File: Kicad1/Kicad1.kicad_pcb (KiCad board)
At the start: 2 copper layers, 12 parts, among them J5 ESP_CONN, J6 ENCODER_CONN, J7 Conn_01x04, U1 STM32F401RBTx, U2 LD1117S50TR_SOT223, U3 LD1117S33TR_SOT223, U4 TB6612FNG, Y1 Crystal_GND24

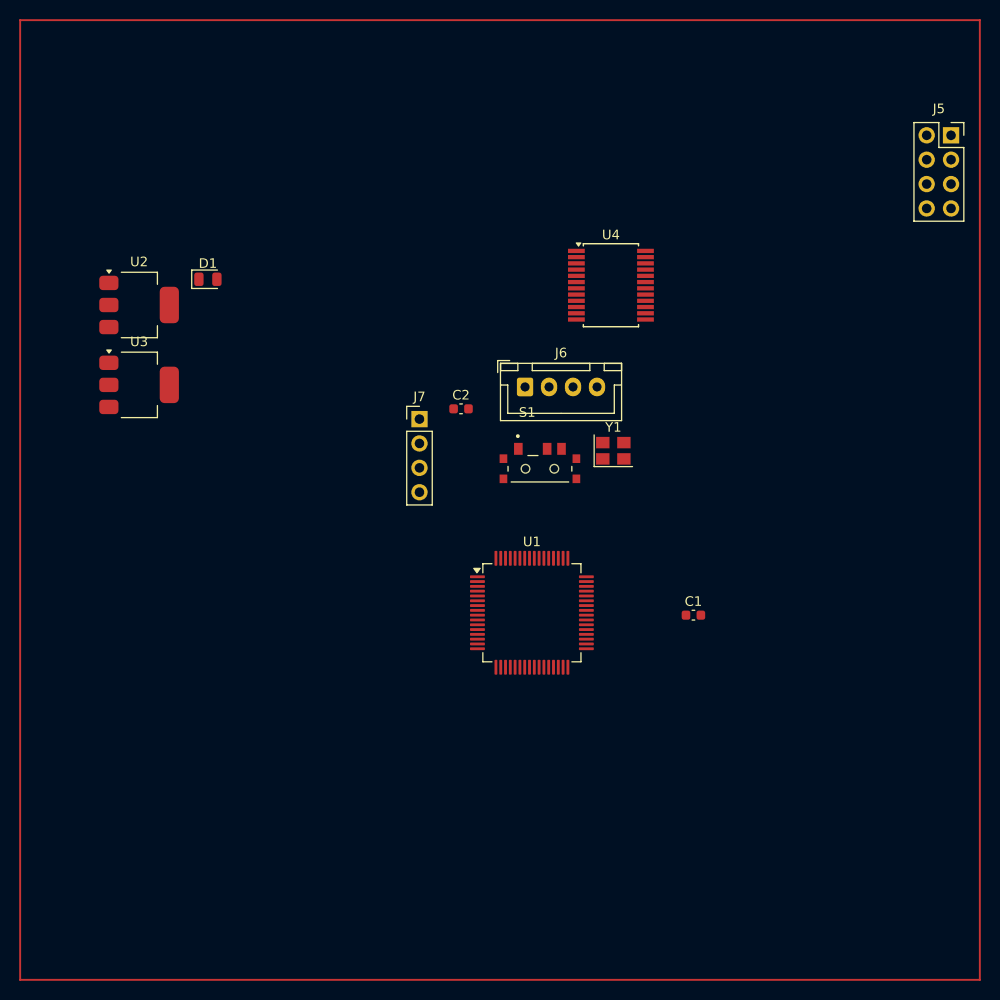
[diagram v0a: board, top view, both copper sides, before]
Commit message: Add files via upload
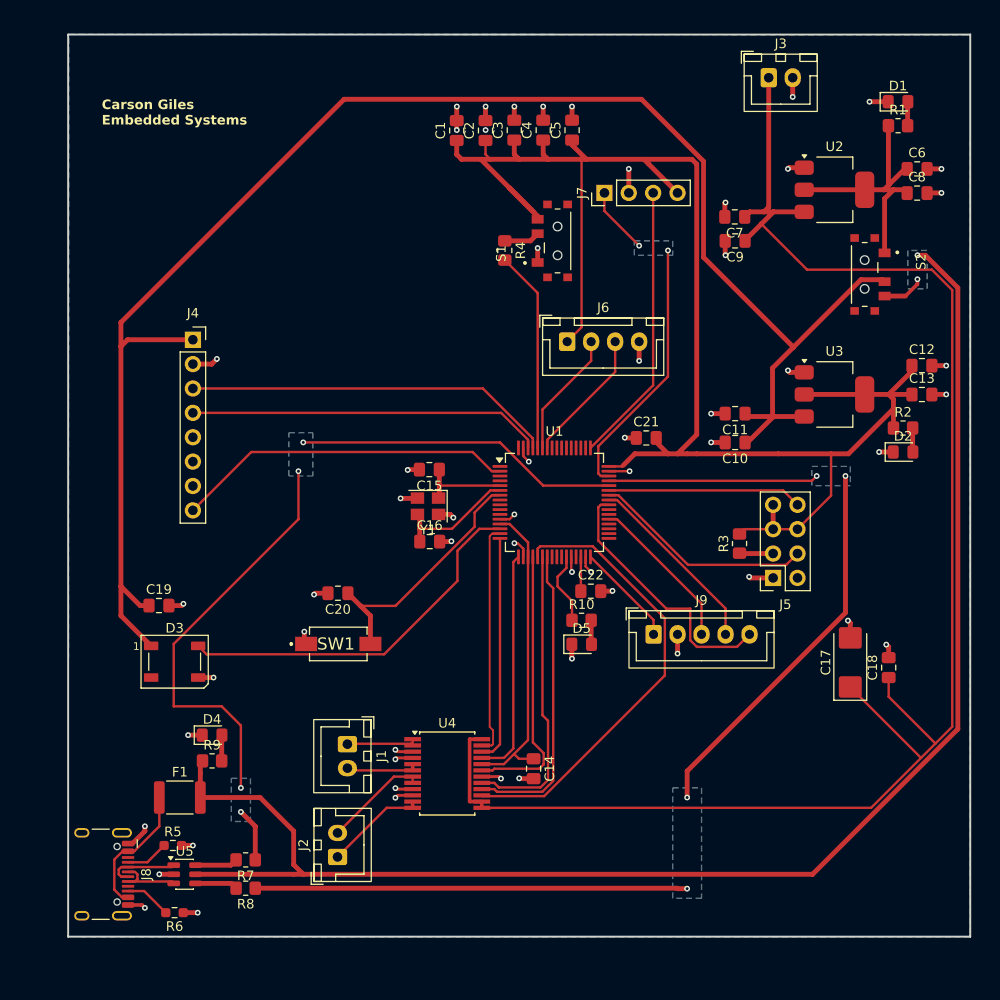
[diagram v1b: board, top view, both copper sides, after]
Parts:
- added C10: 0.1 µF, Capacitor_SMD:C_0805_2012Metric_Pad1.18x1.45mm_HandSolder, F.Cu at (168.5, 81.5)
- added C11: 10 µF, Capacitor_SMD:C_0805_2012Metric_Pad1.18x1.45mm_HandSolder, F.Cu at (168.5, 78.5)
- added C12: 0.1 µF, Capacitor_SMD:C_0805_2012Metric_Pad1.18x1.45mm_HandSolder, F.Cu at (188.0, 73.5)
- added C13: 10 µF, Capacitor_SMD:C_0805_2012Metric_Pad1.18x1.45mm_HandSolder, F.Cu at (188.0, 76.5)
- added C14: 0.1 µF, Capacitor_SMD:C_0805_2012Metric_Pad1.18x1.45mm_HandSolder, F.Cu at (147.5, 115.5)
- added C15: 22 pF, Capacitor_SMD:C_0805_2012Metric_Pad1.18x1.45mm_HandSolder, F.Cu at (136.6, 84.3)
- added C16: 22 pF, Capacitor_SMD:C_0805_2012Metric_Pad1.18x1.45mm_HandSolder, F.Cu at (136.7, 91.8)
- added C17: 10 µF, Capacitor_Tantalum_SMD:CP_EIA-6032-28_Kemet-C_HandSolder, F.Cu at (180.5, 104.4)
- added C18: 0.1 µF, Capacitor_SMD:C_0805_2012Metric_Pad1.18x1.45mm_HandSolder, F.Cu at (184.5, 105.0)
- added C19: 0.1 µF, Capacitor_SMD:C_0805_2012Metric_Pad1.18x1.45mm_HandSolder, F.Cu at (108.5, 98.5)
- added C20: 0.01 µF, Capacitor_SMD:C_0805_2012Metric_Pad1.18x1.45mm_HandSolder, F.Cu at (127.1, 97.2)
- added C21: 0.1 µF, Capacitor_SMD:C_0805_2012Metric_Pad1.18x1.45mm_HandSolder, F.Cu at (159.2, 81.0)
- added C22: 2.2 µF, Capacitor_SMD:C_0805_2012Metric_Pad1.18x1.45mm_HandSolder, F.Cu at (153.5, 97.0)
- added C3: 0.1 µF, Capacitor_SMD:C_0805_2012Metric_Pad1.18x1.45mm_HandSolder, F.Cu at (145.5, 49.0)
- added C4: 0.1 µF, Capacitor_SMD:C_0805_2012Metric_Pad1.18x1.45mm_HandSolder, F.Cu at (148.5, 49.0)
- added C5: 10 µF, Capacitor_SMD:C_0805_2012Metric_Pad1.18x1.45mm_HandSolder, F.Cu at (151.5, 49.0)
- added C6: 0.1 µF, Capacitor_SMD:C_0805_2012Metric_Pad1.18x1.45mm_HandSolder, F.Cu at (187.5, 53.0)
- added C7: 10 µF, Capacitor_SMD:C_0805_2012Metric_Pad1.18x1.45mm_HandSolder, F.Cu at (168.5, 58.0)
- added C8: 10 µF, Capacitor_SMD:C_0805_2012Metric_Pad1.18x1.45mm_HandSolder, F.Cu at (187.5, 55.5)
- added C9: 0.1 µF, Capacitor_SMD:C_0805_2012Metric_Pad1.18x1.45mm_HandSolder, F.Cu at (168.5, 60.5)
- added D2: 3V3_LED, LED_SMD:LED_0805_2012Metric_Pad1.15x1.40mm_HandSolder, F.Cu at (186.0, 82.5)
- added D3: WS2812B, LED_SMD:LED_WS2812B_PLCC4_5.0x5.0mm_P3.2mm, F.Cu at (110.1, 104.3)
- added D4: USB_LED, LED_SMD:LED_0805_2012Metric_Pad1.15x1.40mm_HandSolder, F.Cu at (114.0, 112.0)
- added D5: USER_LED, LED_SMD:LED_0805_2012Metric_Pad1.15x1.40mm_HandSolder, F.Cu at (152.5, 102.5)
- added F1: PTCSMD, Fuse:Fuse_1812_4532Metric, F.Cu at (110.6, 118.5)
- added J1: M1_CONN, Connector_JST:JST_XH_B2B-XH-A_1x02_P2.50mm_Vertical, F.Cu at (128.1, 112.9)
- added J2: M2_CONN, Connector_JST:JST_XH_B2B-XH-A_1x02_P2.50mm_Vertical, F.Cu at (127.1, 124.7)
- added J3: BATT_CONN, Connector_JST:JST_XH_B2B-XH-A_1x02_P2.50mm_Vertical, F.Cu at (172.0, 43.5)
- added J4: Conn_MPU6050, Connector_PinSocket_2.54mm:PinSocket_1x08_P2.54mm_Vertical, F.Cu at (112.0, 70.8)
- added J8: USB_C_Receptacle_USB2.0_14P, Connector_USB:USB_C_Receptacle_HCTL_HC-TYPE-C-16P-01A, F.Cu at (101.5, 126.5)
- added J9: MT6701_CONN, Connector_JST:JST_XH_B5B-XH-A_1x05_P2.50mm_Vertical, F.Cu at (160.0, 101.5)
- added R1: 1 kΩ, Resistor_SMD:R_0805_2012Metric_Pad1.20x1.40mm_HandSolder, F.Cu at (185.5, 48.5)
- added R10: 1 kΩ, Resistor_SMD:R_0805_2012Metric_Pad1.20x1.40mm_HandSolder, F.Cu at (152.5, 100.0)
- added R2: 1 kΩ, Resistor_SMD:R_0805_2012Metric_Pad1.20x1.40mm_HandSolder, F.Cu at (186.0, 80.0)
- added R3: 10K, Resistor_SMD:R_0805_2012Metric_Pad1.20x1.40mm_HandSolder, F.Cu at (169.0, 92.0)
- added R4: 10k, Resistor_SMD:R_0805_2012Metric_Pad1.20x1.40mm_HandSolder, F.Cu at (144.5, 61.5)
- added R5: 5.1 kΩ, Resistor_SMD:R_0603_1608Metric_Pad0.98x0.95mm_HandSolder, F.Cu at (109.9, 123.5)
- added R6: 5.1 kΩ, Resistor_SMD:R_0603_1608Metric_Pad0.98x0.95mm_HandSolder, F.Cu at (110.1, 130.5)
- added R7: 22 Ω, Resistor_SMD:R_0805_2012Metric_Pad1.20x1.40mm_HandSolder, F.Cu at (117.5, 125.0)
- added R8: 22 Ω, Resistor_SMD:R_0805_2012Metric_Pad1.20x1.40mm_HandSolder, F.Cu at (117.5, 128.0)
- added R9: 1 kΩ, Resistor_SMD:R_0805_2012Metric_Pad1.20x1.40mm_HandSolder, F.Cu at (114.0, 114.7)
- added S2: Regulator_Switch, SW_SLW-66527511-SMT-TR:SW_SLW-66527511-SMT-TR, F.Cu at (182.0, 64.0)
- added SW1: SW_UP_Reset, SW_uP_Reset:SW_uP_Reset, F.Cu at (127.2, 102.5)
- added U5: USBLC6-2SC6, Package_TO_SOT_SMD:SOT-23-6, F.Cu at (111.1, 126.5)
- C1, C2: footprint Capacitor_SMD:C_0603_1608Metric -> Capacitor_SMD:C_0805_2012Metric_Pad1.18x1.45mm_HandSolder
- D1: value LED -> 5V_LED; footprint LED_SMD:LED_0805_2012Metric -> LED_SMD:LED_0805_2012Metric_Pad1.15x1.40mm_HandSolder
- S1: value SLW-66527511-SMT-TR -> RST_SWITCH
- Y1: value Crystal_GND24 -> 16MHz
- moved D1 74.3 mm to (185.5, 46.0)
- moved U2 73.4 mm to (178.8, 55.2)
- moved U3 72.5 mm to (178.8, 76.5)
- moved C1 56.2 mm to (139.5, 49.0), turned to 90 degrees
- moved U4 53.7 mm to (138.5, 116.0)
- moved J5 49.7 mm to (172.5, 95.6), turned to 180 degrees
- moved J7 30.4 mm to (154.9, 55.5), turned to 90 degrees
- moved C2 29.1 mm to (142.5, 49.0), turned to 90 degrees
- moved S1 23.8 mm to (150.0, 60.5), turned to 90 degrees
- moved Y1 20.2 mm to (136.5, 88.2), turned to 180 degrees
- moved U1 11.7 mm to (149.7, 87.8)
- moved J6 6.45 mm to (151.0, 71.0)
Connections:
- net Net-(U4-AO1-Pad1) renamed /MD_AO1
- net Net-(U4-AO2-Pad5) renamed /MD_AO2
- net Net-(U4-BO1-Pad11) renamed /MD_BO1
- net Net-(U4-BO2-Pad7) renamed /MD_BO2
- J7 pad 1: /SWDIN -> /SWDIO
- S1 pad 1: unconnected-(S1-Pad1) -> GND
- S1 pad 3: unconnected-(S1-Pad3) -> +3.3V
- U1 pad 12: unconnected-(U1-VSSA-Pad12) -> GND
- U1 pad 13: unconnected-(U1-VREF+-Pad13) -> +3.3V
- U1 pad 14: unconnected-(U1-PA0-Pad14) -> /WS_DIN
- U1 pad 15: unconnected-(U1-PA1-Pad15) -> /MD_PWMA
- U1 pad 16: unconnected-(U1-PA2-Pad16) -> /MD_AIN2
- U1 pad 17: unconnected-(U1-PA3-Pad17) -> /MD_AIN1
- U1 pad 18: Net-(U1-VSS-Pad18) -> GND
- U1 pad 2: unconnected-(U1-PC13-Pad2) -> /IMU_INT
- U1 pad 20: unconnected-(U1-PA4-Pad20) -> /MD_STBY
- U1 pad 21: unconnected-(U1-PA5-Pad21) -> /MD_PWMB
- U1 pad 22: unconnected-(U1-PA6-Pad22) -> /MD_BIN1
- U1 pad 23: unconnected-(U1-PA7-Pad23) -> /MD_BIN2
- U1 pad 27: unconnected-(U1-PB1-Pad27) -> /USER_LED
- U1 pad 28: unconnected-(U1-PB2-Pad28) -> GND
- U1 pad 30: unconnected-(U1-VCAP1-Pad30) -> Net-(U1-VCAP1)
- U1 pad 31: Net-(U1-VSS-Pad18) -> GND
- U1 pad 37: unconnected-(U1-PC6-Pad37) -> /MT_PWM
- U1 pad 40: unconnected-(U1-PC9-Pad40) -> /MT_SDA
- U1 pad 41: unconnected-(U1-PA8-Pad41) -> /MT_SCL
- U1 pad 42: unconnected-(U1-PA9-Pad42) -> /ESP_RX
- U1 pad 43: unconnected-(U1-PA10-Pad43) -> /ESP_TX
- U1 pad 44: unconnected-(U1-PA11-Pad44) -> /ESD_D-
- U1 pad 45: unconnected-(U1-PA12-Pad45) -> /ESD_D+
- U1 pad 46: unconnected-(U1-PA13-Pad46) -> /SWDIO
- U1 pad 47: Net-(U1-VSS-Pad18) -> GND
- U1 pad 49: unconnected-(U1-PA14-Pad49) -> /SWCLK
- U1 pad 58: unconnected-(U1-PB6-Pad58) -> /ENC_B
- U1 pad 59: unconnected-(U1-PB7-Pad59) -> /ENC_A
- U1 pad 61: unconnected-(U1-PB8-Pad61) -> /IMU_SCL
- U1 pad 62: unconnected-(U1-PB9-Pad62) -> /IMU_SDA
- U1 pad 63: Net-(U1-VSS-Pad18) -> GND
- U1 pad 7: unconnected-(U1-NRST-Pad7) -> Net-(SW1A-B)
- U4 pad 10: Net-(U4-PGND2-Pad10) -> GND
- U4 pad 15: unconnected-(U4-PWMB-Pad15) -> /MD_PWMB
- U4 pad 16: unconnected-(U4-BIN2-Pad16) -> /MD_BIN2
- U4 pad 17: unconnected-(U4-BIN1-Pad17) -> /MD_BIN1
- U4 pad 18: unconnected-(U4-GND-Pad18) -> GND
- U4 pad 19: unconnected-(U4-STBY-Pad19) -> /MD_STBY
- U4 pad 21: unconnected-(U4-AIN1-Pad21) -> /MD_AIN1
- U4 pad 22: unconnected-(U4-AIN2-Pad22) -> /MD_AIN2
- U4 pad 23: unconnected-(U4-PWMA-Pad23) -> /MD_PWMA
- U4 pad 3: Net-(U4-PGND1-Pad3) -> GND
- U4 pad 4: Net-(U4-PGND1-Pad3) -> GND
- U4 pad 9: Net-(U4-PGND2-Pad10) -> GND
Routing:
- net +3.3V: track 0.00 -> 219.1 mm
- net VM: track 0.00 -> 174.6 mm
- net +5V: track 0.00 -> 173.9 mm
- net Vusb: track 0.00 -> 161.7 mm, vias 0 -> 2
- net /ESD_D+: track 0.00 -> 107.3 mm, vias 0 -> 4
- net GND: track 0.00 -> 94.1 mm, vias 0 -> 57
- net /ESD_D-: track 0.00 -> 83.5 mm, vias 0 -> 4
- net /MD_PWMB: track 0.00 -> 47.6 mm
- net /WS_DIN: track 0.00 -> 39.1 mm
- net /IMU_SCL: track 0.00 -> 38.6 mm
- net /IMU_SDA: track 0.00 -> 36.9 mm
- net /IMU_INT: track 0.00 -> 35.3 mm
- net /SWDIO: track 0.00 -> 34.5 mm, vias 0 -> 2
- net /MD_BIN2: track 0.00 -> 31.6 mm
- net /MD_BIN1: track 0.00 -> 30.9 mm
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- added copper zone on B.Cu, net /ESD_D+
- added copper zone on B.Cu, net /ESD_D-
- added copper zone on B.Cu, net /SWDIO
- added copper zone on B.Cu, net GND
- added copper zone on B.Cu, net Vusb
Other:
- board outline added: 94 x 94 mm
- board text added: "Carson Giles Embedded Systems"
